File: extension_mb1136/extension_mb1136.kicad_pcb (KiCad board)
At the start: 2 copper layers, 26 parts, among them CN1 Conn_02x19_Odd_Even, CN2 Conn_02x19_Odd_Even, CN3 Conn_01x08, CN4 Conn_01x06, CN5 Conn_01x08, CN6 Conn_01x10, J1 Conn_01x03, J2 Conn_01x03, Q1 S9013, U1 STMPS2151MTR, U2 USBLC6-2

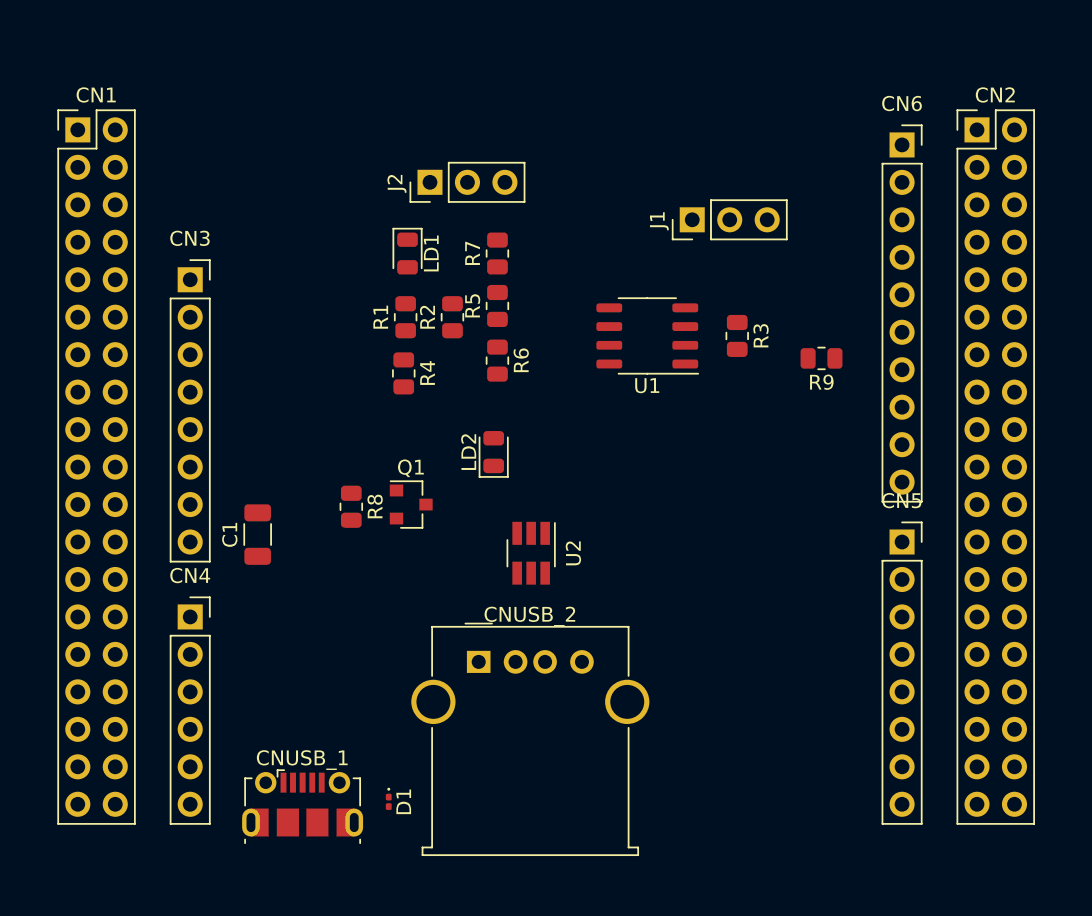
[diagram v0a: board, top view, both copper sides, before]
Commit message: add connector, develop pcb
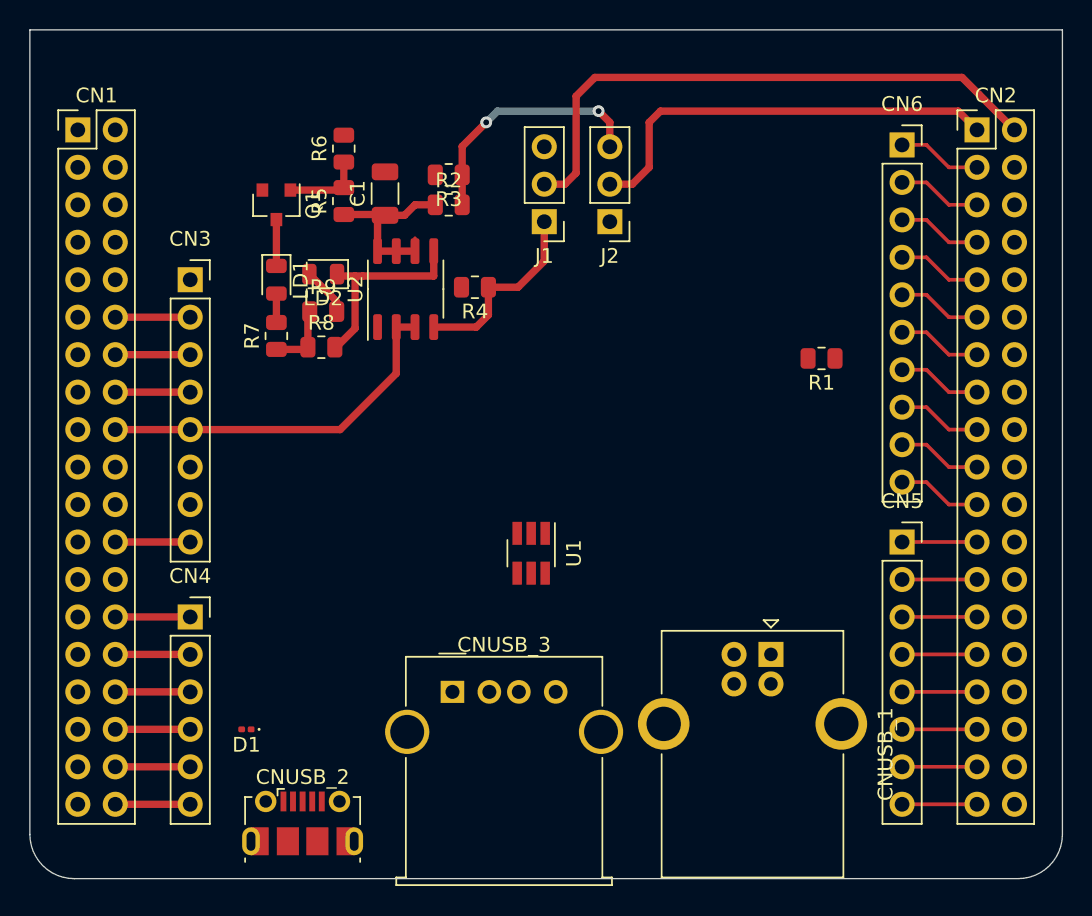
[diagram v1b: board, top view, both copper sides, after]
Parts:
- added CNUSB_1: USB_B, Connector_USB:USB_B_OST_USB-B1HSxx_Horizontal, F.Cu at (72.4, 88.9)
- moved C1 24.7 mm to (46.2, 57.7)
- moved R6 24.3 mm to (43.4, 54.6), turned to 90 degrees
- moved Q1 22.3 mm to (38.9, 58.4), turned to 270 degrees
- moved LD1 18.8 mm to (38.9, 63.5), turned to 270 degrees
- moved R4 18.1 mm to (52.3, 64.0), turned to 180 degrees
- moved U2 16.7 mm to (47.6, 64.1), turned to 90 degrees
- moved R5 15.0 mm to (43.4, 58.2), turned to 90 degrees
- moved J2 12.5 mm to (61.5, 59.6), turned to 180 degrees
- moved D1 10.8 mm to (36.8, 94.0), turned to 180 degrees
- moved J1 10.0 mm to (57.0, 59.6), turned to 180 degrees
- moved R8 9.12 mm to (41.9, 68.1), turned to 0 degrees
- moved R7 9.00 mm to (38.9, 67.3), turned to 90 degrees
- moved R2 7.61 mm to (50.5, 58.4), turned to 0 degrees
- moved R3 6.27 mm to (50.5, 56.4), turned to 180 degrees
- moved LD2 5.88 mm to (42.0, 63.1), turned to 180 degrees
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- renumbered CNUSB_1 to CNUSB_2, CNUSB_2 to CNUSB_3, LD2 to LD1, LD1 to LD2, R9 to R1, R5 to R2, R7 to R3, R3 to R4, R6 to R5, R8 to R6, R4 to R7, R2 to R8, R1 to R9, U2 to U1, U1 to U2
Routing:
- net PC8: track 0.00 -> 39.4 mm
- net PC9: track 0.00 -> 29.3 mm
- net +5V: track 0.00 -> 25.0 mm
- net PA9: track 0.00 -> 18.5 mm
- net VBUS_DET: track 0.00 -> 17.1 mm, vias 0 -> 2
- net USB_OWER_CURRENT: track 0.00 -> 13.7 mm
- net USB_POWER_SWITCH_ON: track 0.00 -> 13.1 mm
- net +3V3: track 0.00 -> 9.74 mm
- net PA7: track 0.00 -> 5.71 mm
- net PA5: track 0.00 -> 5.71 mm
- net PB9: track 0.00 -> 5.71 mm
- net PB8: track 0.00 -> 5.71 mm
- net GND: track 0.00 -> 5.71 mm
- net AVDD: track 0.00 -> 5.71 mm
- net PC7: track 0.00 -> 5.71 mm
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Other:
- board outline added: 70 x 57.5 mm
